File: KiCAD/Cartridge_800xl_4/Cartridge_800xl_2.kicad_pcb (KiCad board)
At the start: 4 copper layers, 64 x 82.6 mm, 21 parts, among them SW1 Reset, U1 27C512, U2 74HC165, U3 74HC595, U4 GAL16V8, U5 TXS0108EPW, U6 mini_esp32

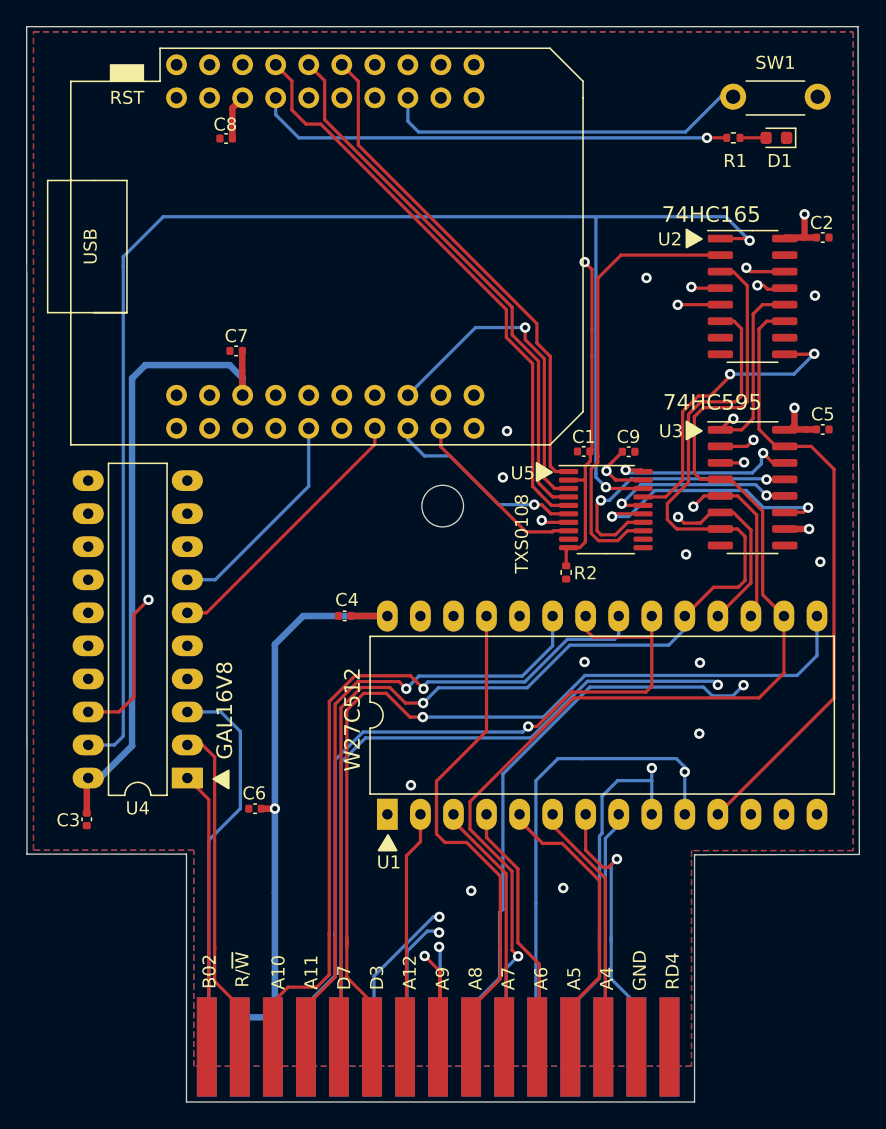
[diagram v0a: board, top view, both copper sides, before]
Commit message: pcb update
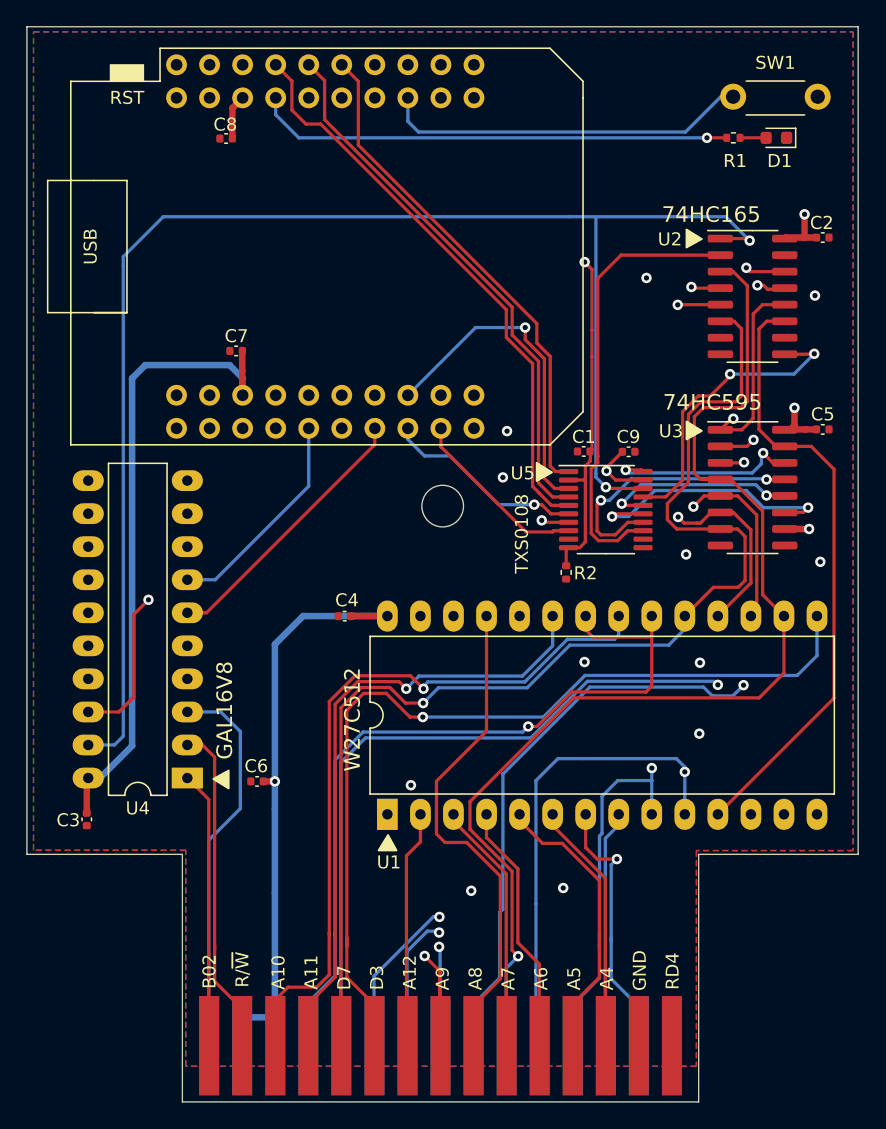
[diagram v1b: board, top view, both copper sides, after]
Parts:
- C1, C3, C4, C5, C6, C7, C8, C9: value 100n -> 100nF
- D1: value LED -> LED red
- R2: value 10k -> 10kΩ
- moved C6 2.10 mm to (137.4, 118.2)
- moved Z1 0.21 mm to (133.9, 138.7)
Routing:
- net +5V: track 201.6 -> 202.3 mm
- net A3: track 21.7 -> 21.0 mm
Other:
- board size 64 x 82.6 mm -> 63.9 x 82.6 mm
